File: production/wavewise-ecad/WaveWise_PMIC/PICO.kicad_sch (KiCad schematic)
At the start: 1 part, among them U1 Raspberry Pi Pico

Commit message: added most footprints still need polulu footprint
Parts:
- U1: footprint RPi_Pico:RPi_Pico_SMD_TH -> Unchecked:Pico
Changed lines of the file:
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@@
       (effects (font (size 1.27 1.27)))
     )
-    (property "Footprint" "RPi_Pico:RPi_Pico_SMD_TH" (at 58.928 48.006 90)
+    (property "Footprint" "Unchecked:Pico" (at 58.928 48.006 90)
       (effects (font (size 1.27 1.27)) hide)
     )

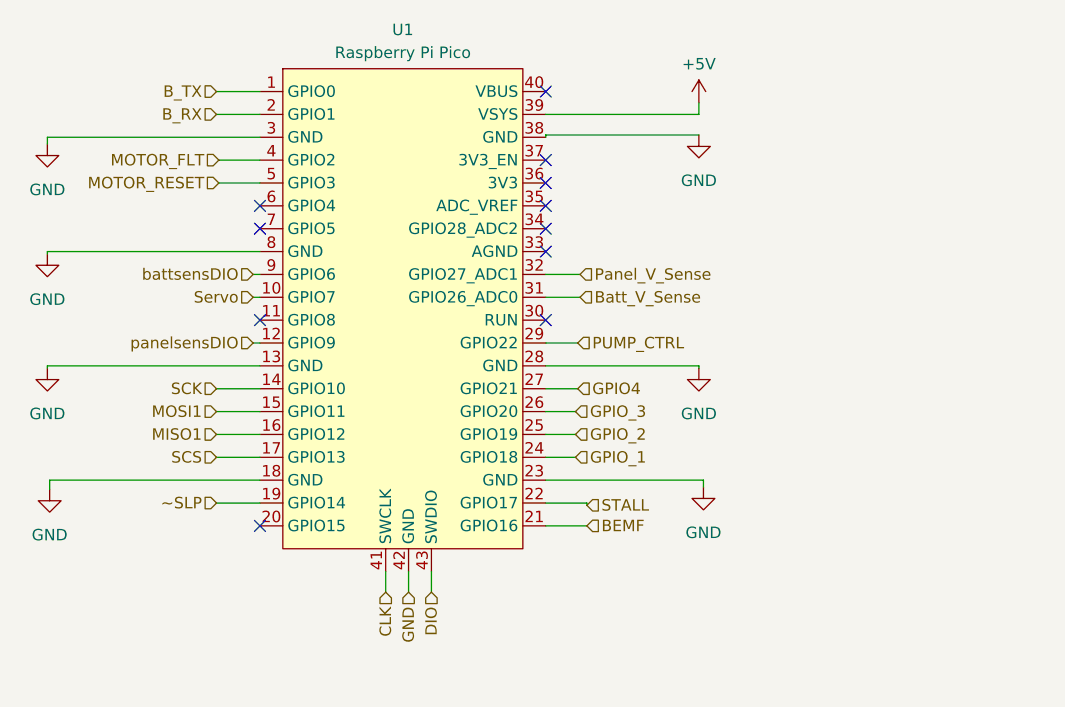
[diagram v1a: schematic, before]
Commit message: Prelim board layout
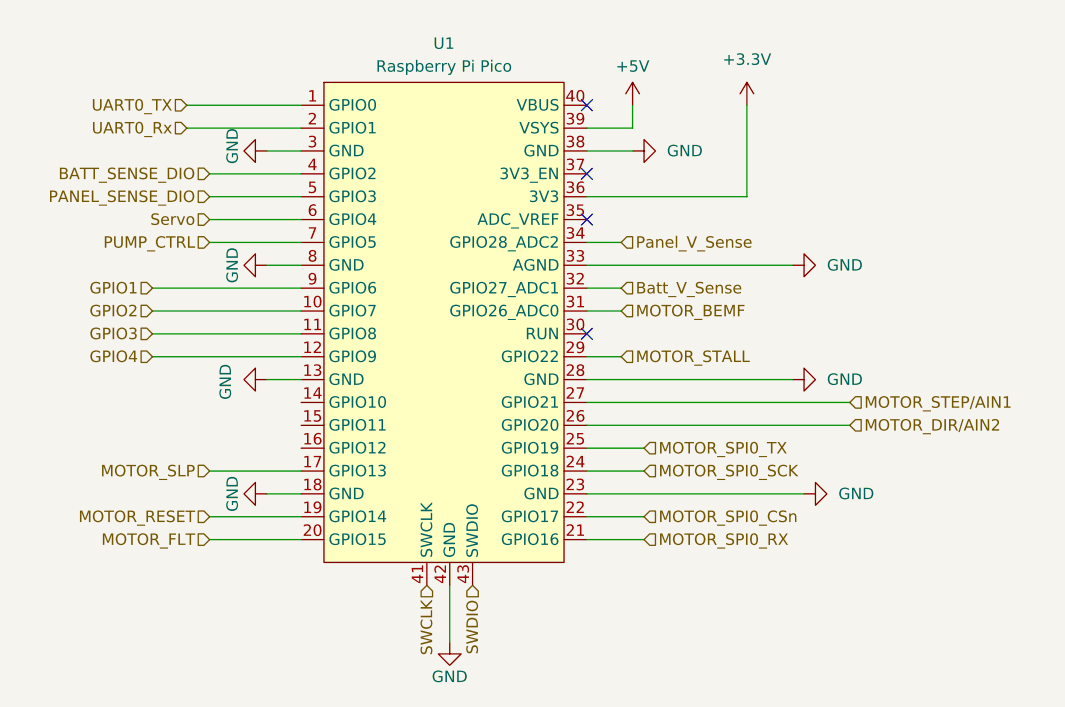
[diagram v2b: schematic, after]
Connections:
- net panelsensDIO is gone; now on net GPIO4: U1.12 (GPIO9)
- net ~SLP is gone; now on net MOTOR_RESET: U1.19 (GPIO14)
- net Batt_V_Sense: now also U1.32 (GPIO27_ADC1); no longer U1.31 (GPIO26_ADC0)
- net GND: now also U1.33 (AGND)
- net GPIO4: no longer U1.27 (GPIO21)
- net MOTOR_FLT: now also U1.20 (GPIO15); no longer U1.4 (GPIO2)
- net MOTOR_RESET: no longer U1.5 (GPIO3)
- net PUMP_CTRL: now also U1.7 (GPIO5); no longer U1.29 (GPIO22)
- net Panel_V_Sense: now also U1.34 (GPIO28_ADC2); no longer U1.32 (GPIO27_ADC1)
- net Servo: now also U1.6 (GPIO4); no longer U1.10 (GPIO7)
- net GPIO3: now reaches U1.11 (GPIO8)
- net +3.3V: now reaches U1.36 (3V3)
- net BEMF renamed MOTOR_SPI0_RX
- net B_RX renamed UART0_Rx
- net B_TX renamed UART0_TX
- net CLK renamed SWCLK
- net DIO renamed SWDIO
- net GPIO_1 renamed MOTOR_SPI0_SCK
- net GPIO_2 renamed MOTOR_SPI0_TX
- net GPIO_3 renamed MOTOR_DIR/AIN2
- net MISO1: no longer names the net of U1.16 (GPIO12)
- net MOSI1: no longer names the net of U1.15 (GPIO11)
- net SCK: no longer names the net of U1.14 (GPIO10)
- net SCS renamed MOTOR_SLP
- net STALL renamed MOTOR_SPI0_CSn
- net battsensDIO renamed GPIO1
- new net BATT_SENSE_DIO: U1.4 (GPIO2)
- new net GPIO2: U1.10 (GPIO7)
- new net MOTOR_BEMF: U1.31 (GPIO26_ADC0)
- new net MOTOR_STALL: U1.29 (GPIO22)
- new net MOTOR_STEP/AIN1: U1.27 (GPIO21)
- new net PANEL_SENSE_DIO: U1.5 (GPIO3)
- no-connect marks 11 -> 4
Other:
- moved on the sheet: U1
